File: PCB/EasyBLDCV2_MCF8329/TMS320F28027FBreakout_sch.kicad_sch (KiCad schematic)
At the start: 25 parts, among them J2 Conn_01x16_Pin, U1 MCF8329A1IREER

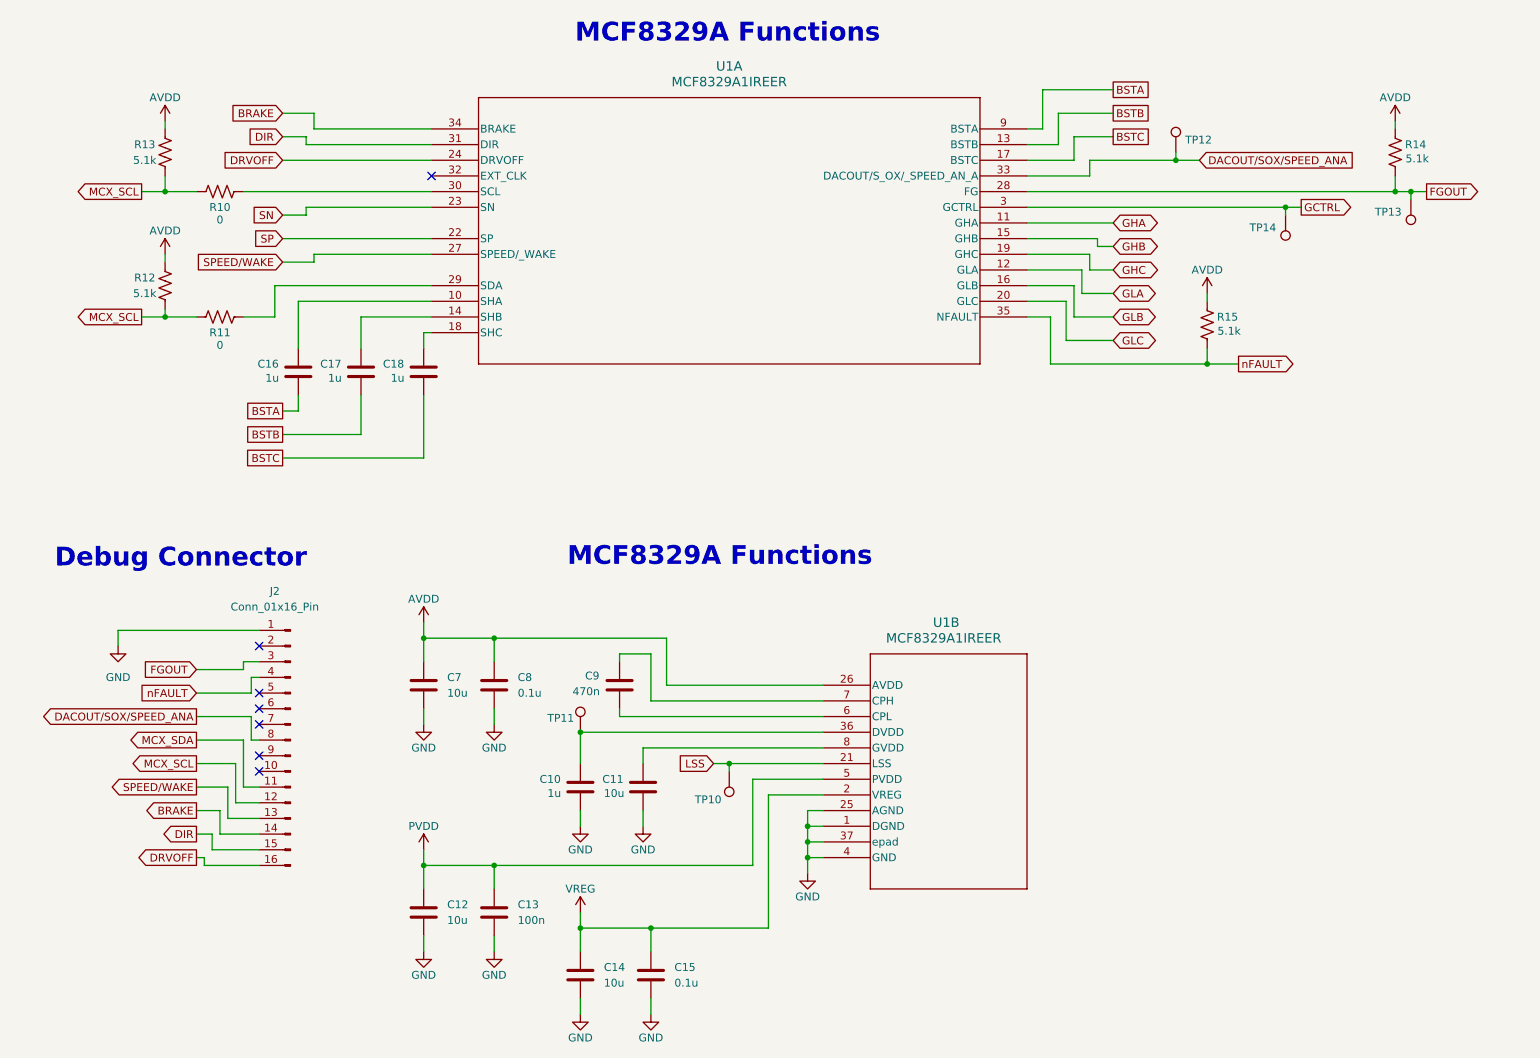
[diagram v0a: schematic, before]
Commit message: Finished schematic
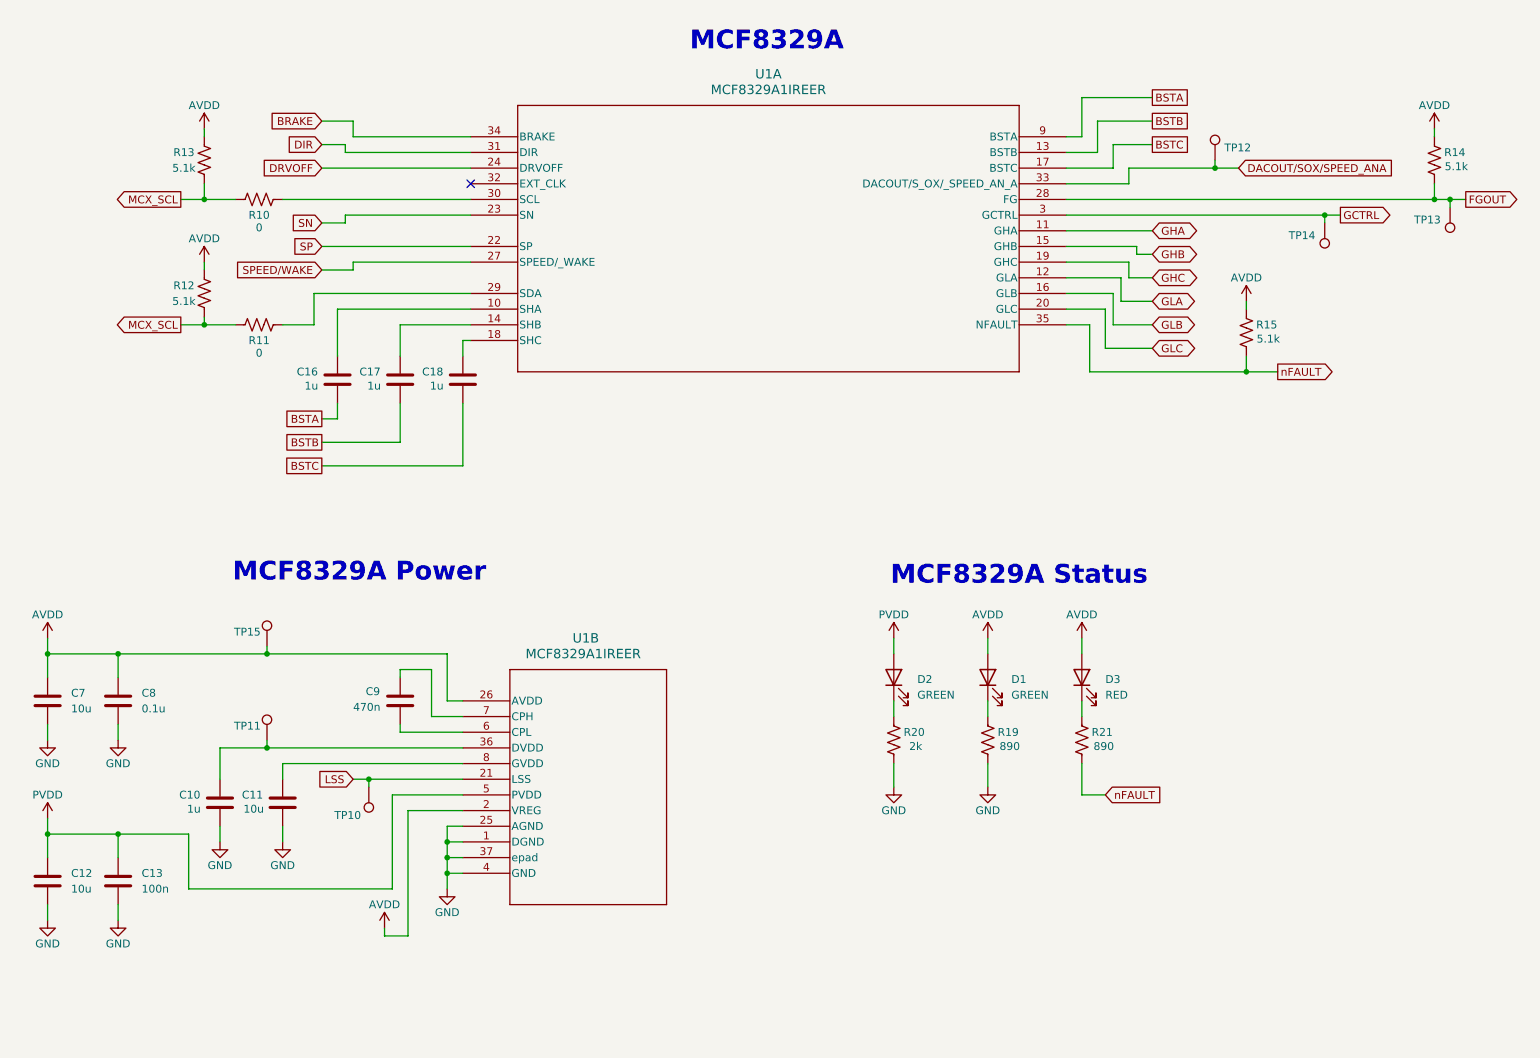
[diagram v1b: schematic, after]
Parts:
- removed C14: 10u, symbol Device:C
- removed C15: 0.1u, symbol Device:C
- removed J2: Conn_01x16_Pin, symbol Connector:Conn_01x16_Pin
- added D1, D2: GREEN, symbol Device:LED
- added D3: RED, symbol Device:LED
- added R19, R21: 890, symbol Device:R_US
- added R20: 2k, symbol Device:R_US
- added TP15: TestPoint, symbol Connector:TestPoint
- R10, R11, R12, R13, R14, R15: footprint Resistor_SMD:R_2512_6332Metric -> (none)
- U1: footprint WQFN36_REE_TEX -> EasyBLDC:WQFN36_REE_TEX
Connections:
- net VREG is gone; now on net AVDD: U1.2 (VREG)
- net AVDD: now also D1.2 (A), D3.2 (A), TP15.1
- net GND: now also R19.1, R20.1
- net PVDD: now also D2.2 (A)
- net nFAULT: now also R21.1
- new net: D2.1 (K), R20.2
- new net: D1.1 (K), R19.2
- new net: D3.1 (K), R21.2
- no-connect marks 7 -> 1
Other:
- note added: "MCF8329A"
- note added: "MCF8329A Power"
- note added: "MCF8329A Status"
- note removed: "Debug Connector"
- note removed: "MCF8329A Functions"
- moved on the sheet: C10, C11, C12, C13, C16, C17, C18, C7, C8, C9, R10, R11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
